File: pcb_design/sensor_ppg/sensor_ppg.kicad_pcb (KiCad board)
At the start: 2 copper layers, 15 x 23 mm, 12 parts, among them J1 Conn_01x07_Pin, U1 MAX30102EFD_T, U2 MIC5365-1.8YMT-TZ

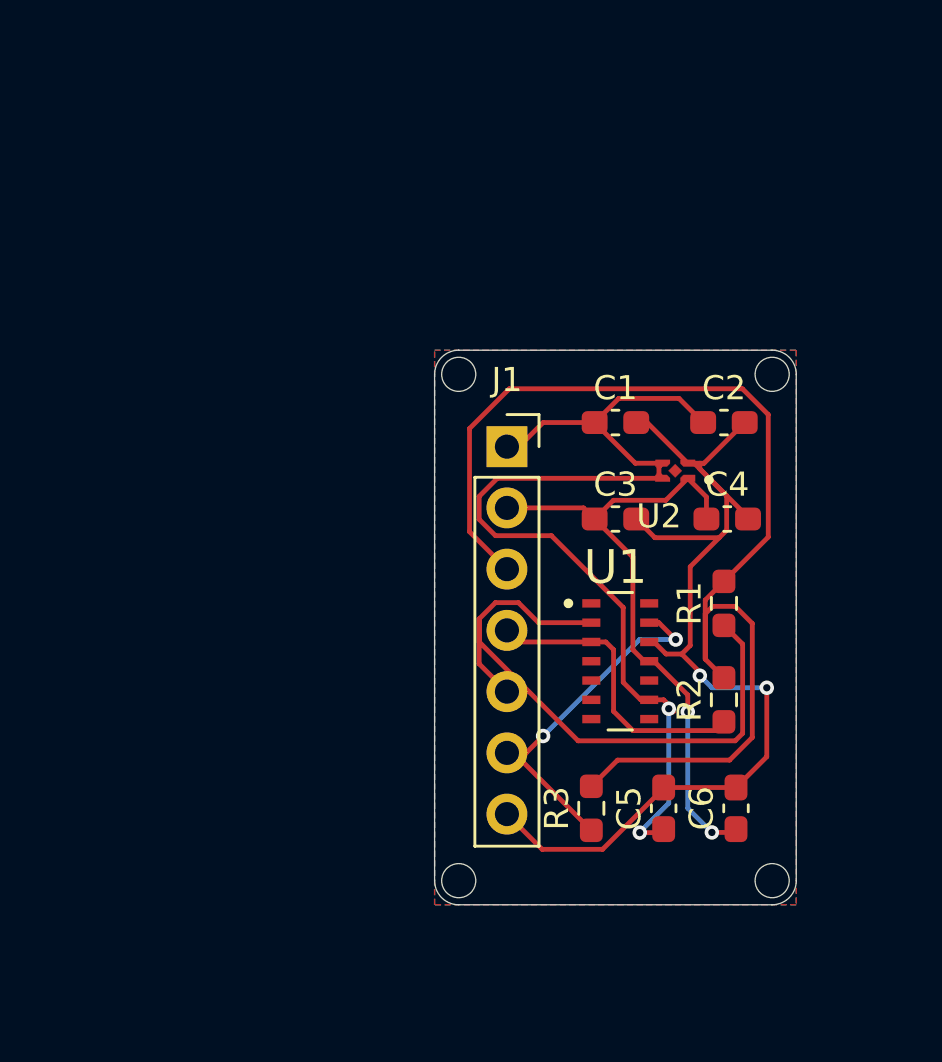
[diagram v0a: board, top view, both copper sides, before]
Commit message: update pcb, cad, and code
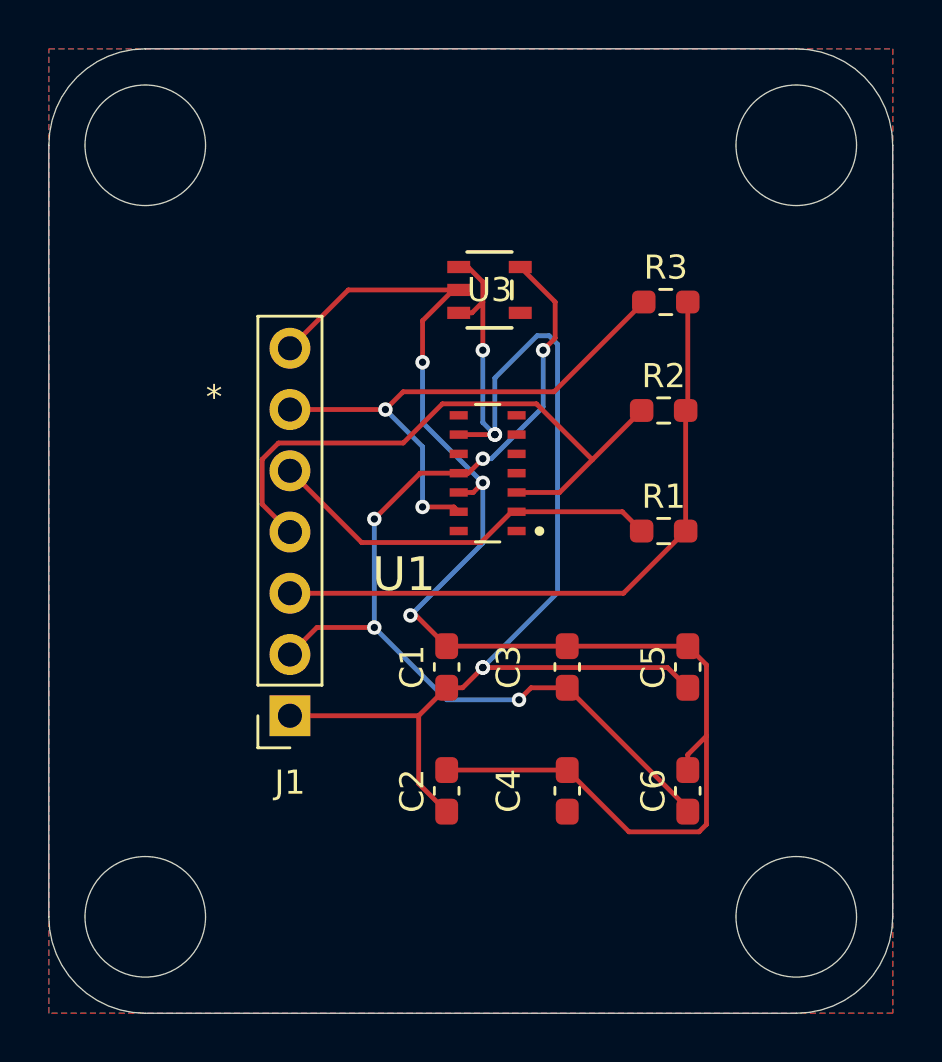
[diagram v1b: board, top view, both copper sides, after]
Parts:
- removed U2: MIC5365-1.8YMT-TZ, MIC5365_1_8YMT_TZ_snap:VREG_MIC5365-1.8YMT-TZ
- added U3: MIC5365-1.8YD5-TR, MIC5365_1_8YD5_TR:TSOT-23-5_D5_MCH, F.Cu at (123.3, 75.0)
- moved R3 21.2 mm to (130.6, 75.5), turned to 0 degrees
- moved C2 19.1 mm to (121.5, 95.8), turned to 90 degrees
- moved J1 14.3 mm to (115.0, 92.7), turned to 180 degrees
- moved C4 13.1 mm to (126.5, 95.8), turned to 90 degrees
- moved C1 12.3 mm to (121.5, 90.6), turned to 90 degrees
- moved R2 12.3 mm to (130.5, 80.0), turned to 0 degrees
- moved U1 9.54 mm to (123.2, 82.6), turned to 180 degrees
- moved C3 6.46 mm to (126.5, 90.6), turned to 90 degrees
- moved C5 5.95 mm to (131.5, 90.6)
- moved R1 3.91 mm to (130.5, 85.0), turned to 0 degrees
- moved C6 2.13 mm to (131.5, 95.8)
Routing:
- net /VDDIO: track 48.8 -> 27.0 mm
- net GND: track 43.9 -> 59.1 mm, vias 2 -> 3
- net +1V8: track 26.7 -> 40.7 mm, vias 2 -> 5
- net /SDA: track 12.4 -> 25.7 mm
- net /SCL: track 27.3 -> 16.7 mm
- net +3.3V: track 42.7 -> 53.2 mm, vias 2 -> 5
- net /INT: track 15.2 -> 23.0 mm
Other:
- board size 15 x 23 mm -> 35 x 40 mm
